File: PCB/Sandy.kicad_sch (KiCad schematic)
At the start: 151 parts, among them J1 USB_C_Receptacle_USB2.0, J10 Conn_02x02_Top_Bottom, J2 Conn_01x03, J3 Conn_01x02, J4 Conn_02x03_Odd_Even, J5 Conn_02x02_Top_Bottom, J6 Conn_02x02_Top_Bottom, J7 Conn_02x02_Top_Bottom, J8 Conn_02x02_Top_Bottom, J9 Conn_02x02_Top_Bottom, U1 ATmega32U4-MU, U2 24LC64, Y1 16MHz

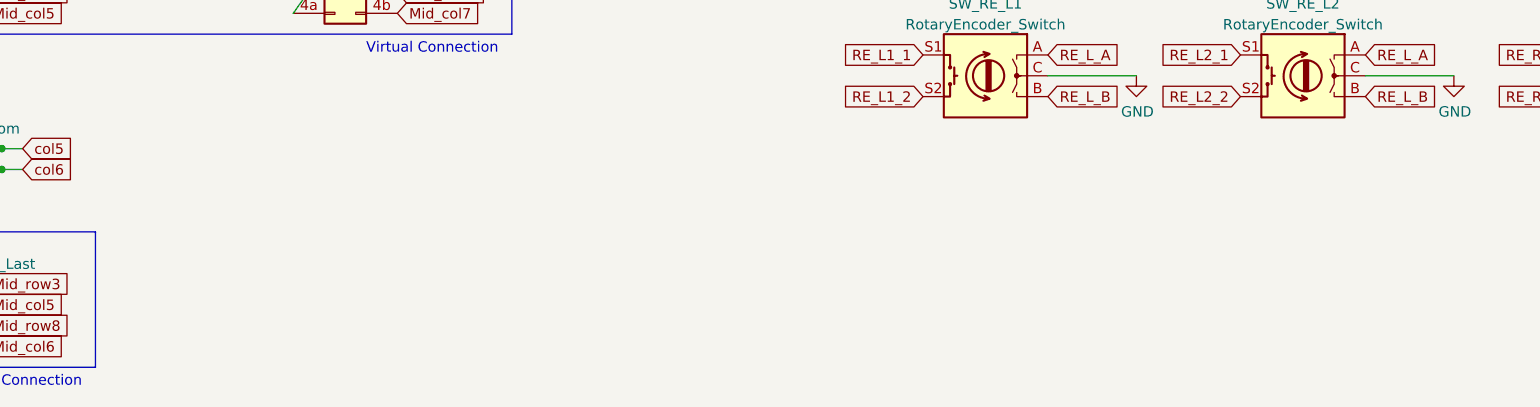
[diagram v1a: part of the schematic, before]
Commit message: JSTコネクタとスペーサーでなんとするテスト
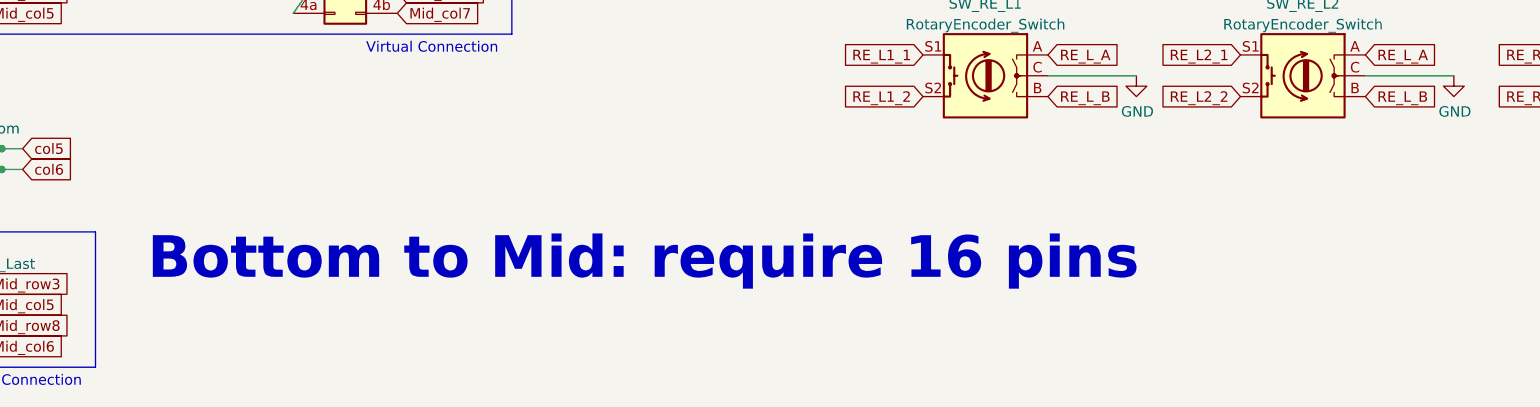
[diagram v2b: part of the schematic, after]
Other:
- note added: "Bottom to Mid: require 16 pins"
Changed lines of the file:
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@@
     (effects (font (size 1.27 1.27)) (justify left bottom))
   )
+  (text "Bottom to Mid: require 16 pins" (at 165.1 271.78 0)
+    (effects (font (size 5.08 5.08) (thickness 1.016) bold) (justify left bottom))
+  )
   (text "Panel CONNECTOR\nBase to Middle" (at 15.24 208.28 0)
     (effects (font (size 2.54 2.54) (thickness 0.508) bold) (justify left bottom))
@@
       (reference "D59") (unit 1) (value "D") (footprint "Diode_SMD:D_SOD-123")
     )
+    (path "/657e3a5b-6fed-49ab-8642-9fbc0b768079/73f1126e-ca87-4e09-a1ed-b765b426e7b4"
+      (reference "D60") (unit 1) (value "D") (footprint "Diode_SMD:D_SOD-123")
+    )
+    (path "/657e3a5b-6fed-49ab-8642-9fbc0b768079/ea2e9c6d-5ae0-42fe-a35c-3b7710e3ca82"
+      (reference "D61") (unit 1) (value "D") (footprint "Diode_SMD:D_SOD-123")
+    )
+    (path "/657e3a5b-6fed-49ab-8642-9fbc0b768079/96c16827-6231-4530-b5c3-beed48e5205b"
+      (reference "D62") (unit 1) (value "D") (footprint "Diode_SMD:D_SOD-123")
+    )
+    (path "/657e3a5b-6fed-49ab-8642-9fbc0b768079/74555395-ef4f-4df9-aa65-ba6e2cd5ce99"
+      (reference "D63") (unit 1) (value "D") (footprint "Diode_SMD:D_SOD-123")
+    )
+    (path "/657e3a5b-6fed-49ab-8642-9fbc0b768079/f4f6b2f4-47ed-4341-a133-b7eea3e6b0a6"
+      (reference "D64") (unit 1) (value "D") (footprint "Diode_SMD:D_SOD-123")
+    )
     (path "/00000000-0000-0000-0000-00005f65b38d"
       (reference "D74") (unit 1) (value "D") (footprint "Diode_SMD:D_SOD-123")
@@
     )
     (path "/657e3a5b-6fed-49ab-8642-9fbc0b768079/4e814551-707a-49cd-a5cf-4a7c6dde6d6c"
-      (reference "S?") (unit 1) (value "JS5208") (footprint "SW_JS5208")
+      (reference "S1") (unit 1) (value "JS5208") (footprint "locallib:SW_JS5208_add_MP_hole")
+    )
+    (path "/657e3a5b-6fed-49ab-8642-9fbc0b768079/f19acb18-ba6b-4e84-8e72-30eac013a8b9"
+      (reference "S2") (unit 1) (value "JS5208") (footprint "locallib:SW_JS5208_add_MP_hole")
     )
     (path "/657e3a5b-6fed-49ab-8642-9fbc0b768079/9b60bbe6-6e78-46e7-aacd-e2e4b03eb7ba"
